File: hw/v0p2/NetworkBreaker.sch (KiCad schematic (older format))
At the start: 32 parts, among them J1 8P8C_Shielded, J2 8P8C_Shielded, J3 8P8C_Shielded, K1 M4-5HAW, K2 M4-5HAW, K3 M4-5HAW, K4 M4-5HAW, Q1 2N3904, Q2 2N3904, Q3 2N3904, Q4 2N3904, U1 TLP627-4

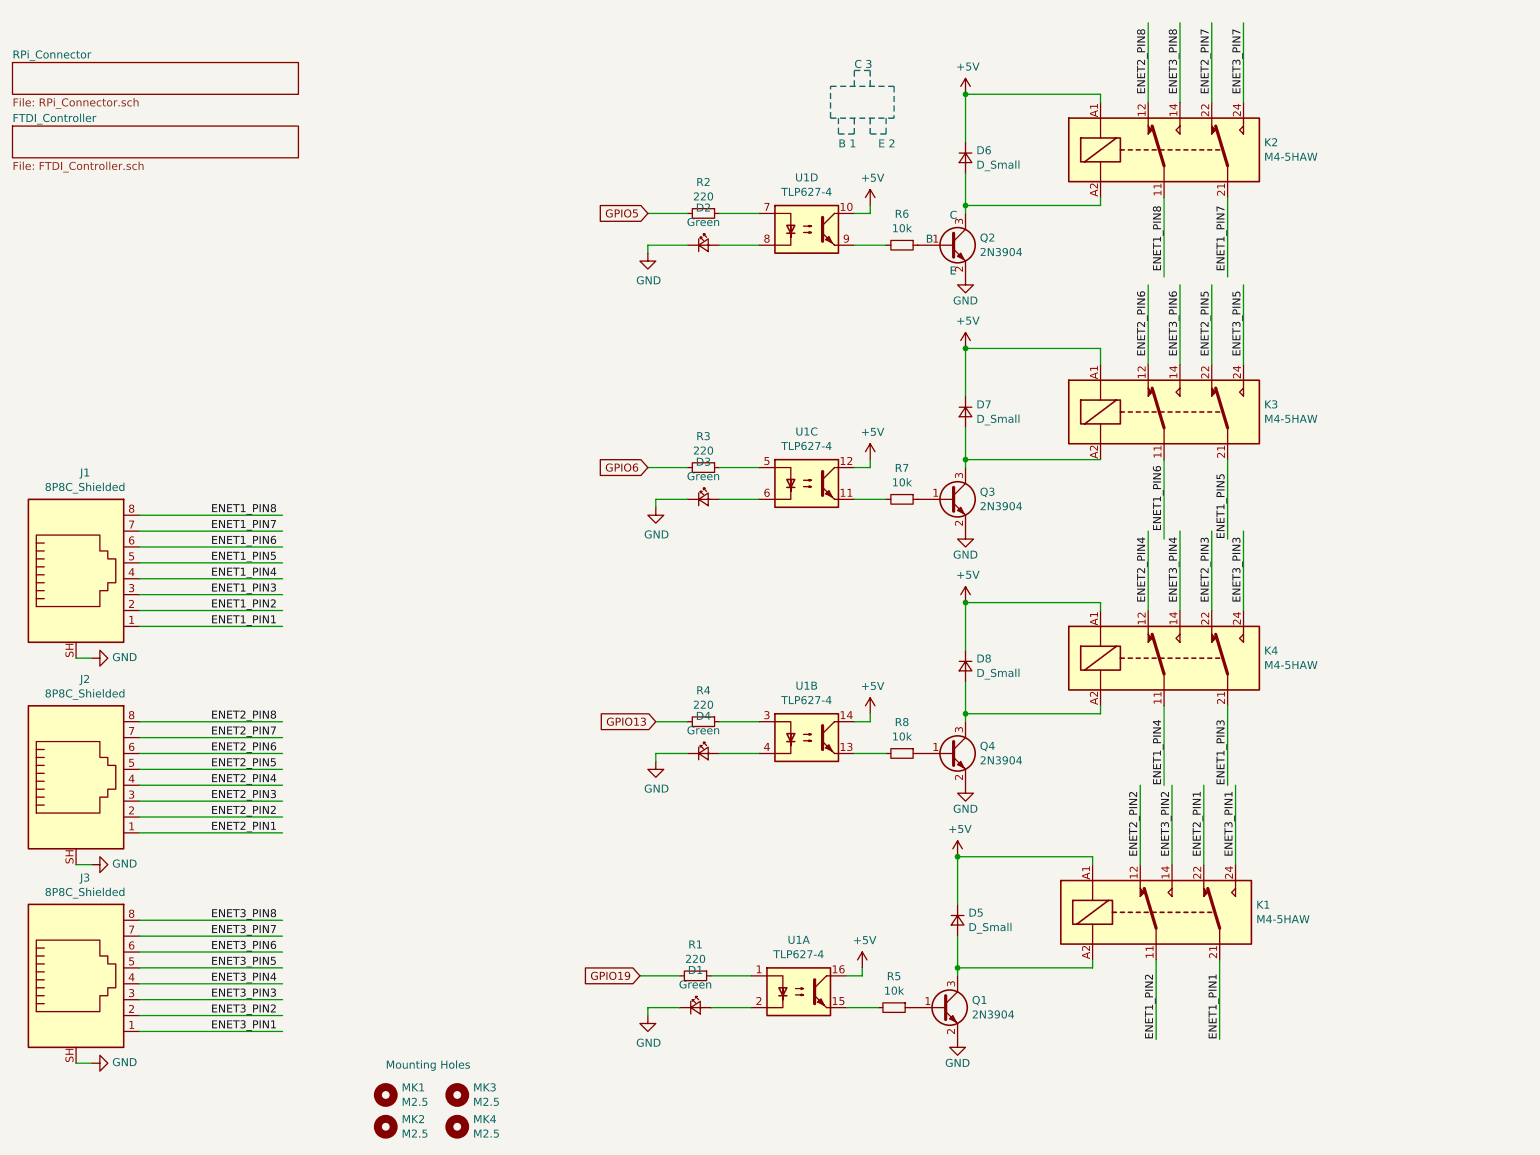
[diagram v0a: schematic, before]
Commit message: Updated
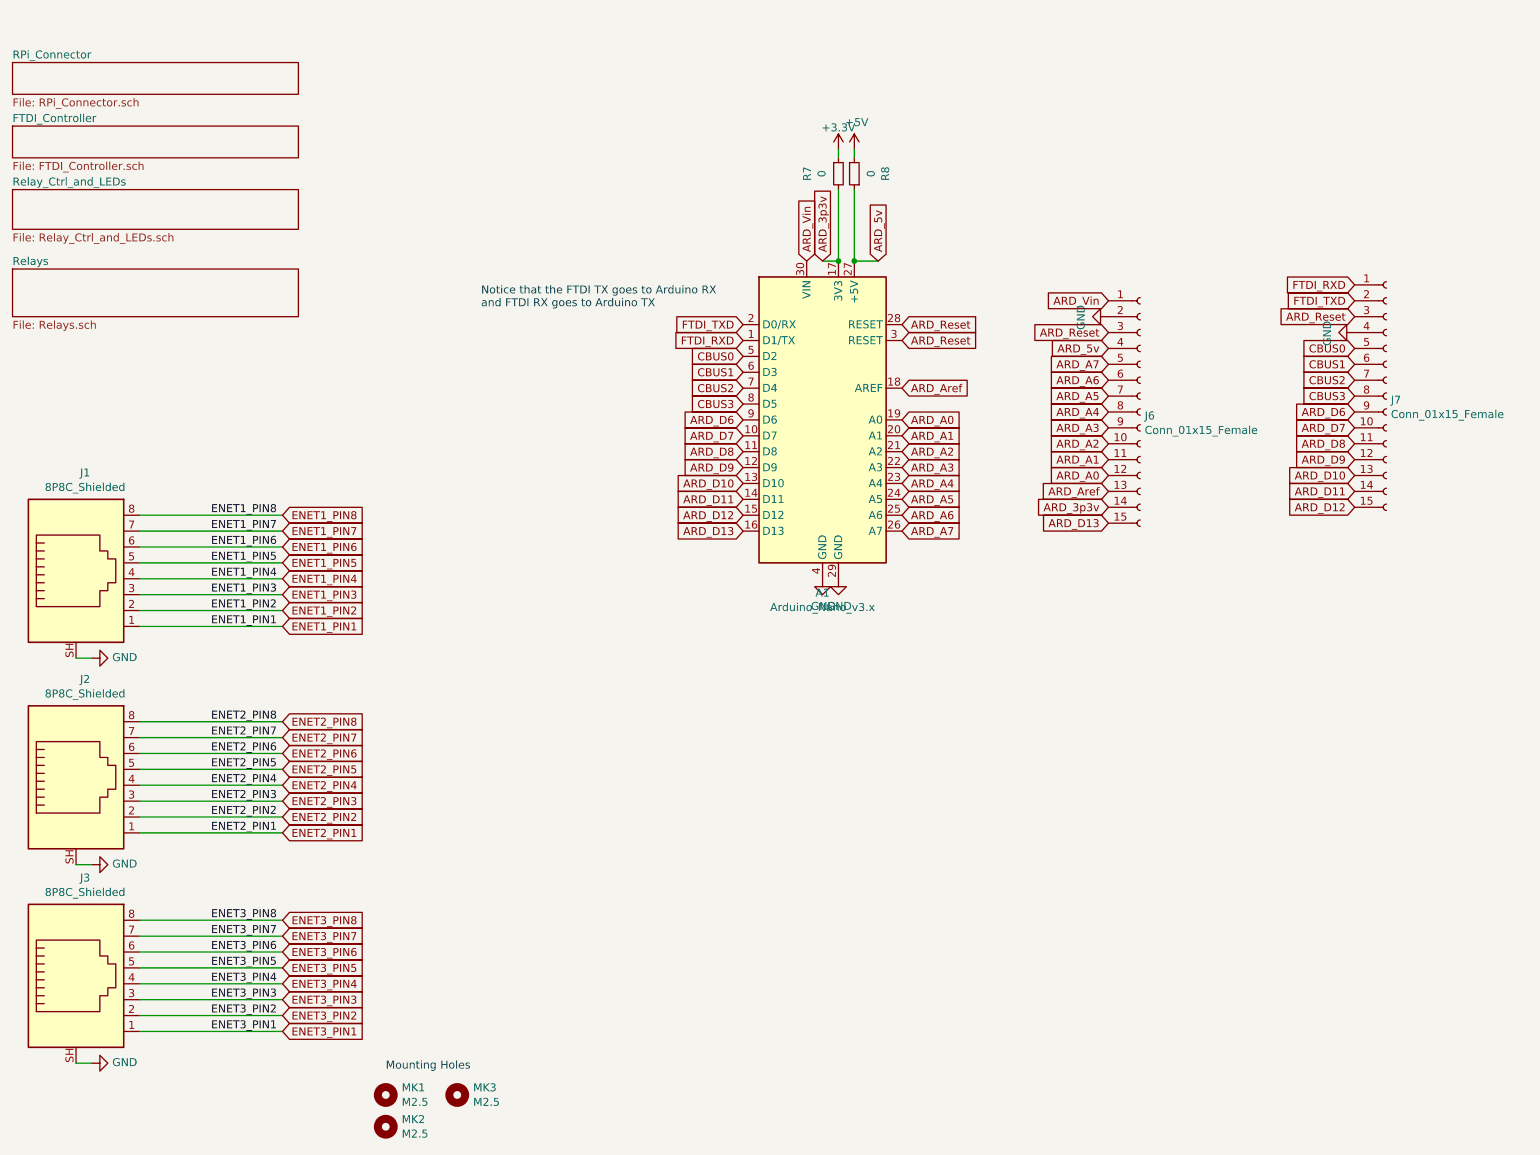
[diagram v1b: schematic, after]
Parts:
- removed D1, D2, D3, D4: Green, LED_SMD:LED_0805_2012Metric, symbol Device:LED_Small
- removed D5, D6, D7, D8: D_Small, Diode_SMD:D_SOD-123F, symbol Device:D_Small
- removed K1, K2, K3, K4: M4-5HAW, Relay_THT:Relay_DPDT_Finder_30.22, symbol Relay:FINDER-30.22
- removed MK4: M2.5, MountingHole:MountingHole_2.7mm_M2.5, symbol NetworkBreaker-rescue:Mounting_Hole-Mechanical
- removed Q1, Q2, Q3, Q4: 2N3904, Package_TO_SOT_SMD:SOT-23, symbol Transistor_BJT:BC818
- removed R1, R2, R3, R4: 220, Resistor_SMD:R_0805_2012Metric, symbol Device:R_Small
- removed R5, R6: 10k, Resistor_SMD:R_0805_2012Metric, symbol Device:R_Small
- removed U1: TLP627-4, Package_DIP:DIP-16_W7.62mm, symbol Isolator:LTV-847M
- added A1: Arduino_Nano_v3.x, Module:Arduino_Nano, symbol MCU_Module:Arduino_Nano_v3.x
- added J6, J7: Conn_01x15_Female, Connector_PinSocket_2.54mm:PinSocket_1x15_P2.54mm_Vertical, symbol Connector:Conn_01x15_Female
- R7, R8: value 10k -> 0; LCSC C180849 -> C17477
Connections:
- net labels added: +3.3V, ARD_3p3v, ARD_5v, ARD_A0, ARD_A1, ARD_A2, ARD_A3, ARD_A4, ARD_A5, ARD_A6, ARD_A7, ARD_Aref, ARD_D10, ARD_D11, ARD_D12, ARD_D13, ARD_D6, ARD_D7, ARD_D8, ARD_D9, ARD_Reset, ARD_Vin, CBUS0, CBUS1, CBUS2, CBUS3, FTDI_RXD, FTDI_TXD
- net labels removed: GPIO13, GPIO19, GPIO5, GPIO6
- wire segments 110 -> 33
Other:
- note added: "Notice that the FTDI TX goes to Arduino RX\nand FTDI RX goes to Arduino TX"
- note removed: "B"
- note removed: "B 1"
- note removed: "C"
- note removed: "C 3"
- note removed: "E"
- note removed: "E 2"
